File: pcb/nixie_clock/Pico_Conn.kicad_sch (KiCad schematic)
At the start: 1 part, among them U14 PicoW

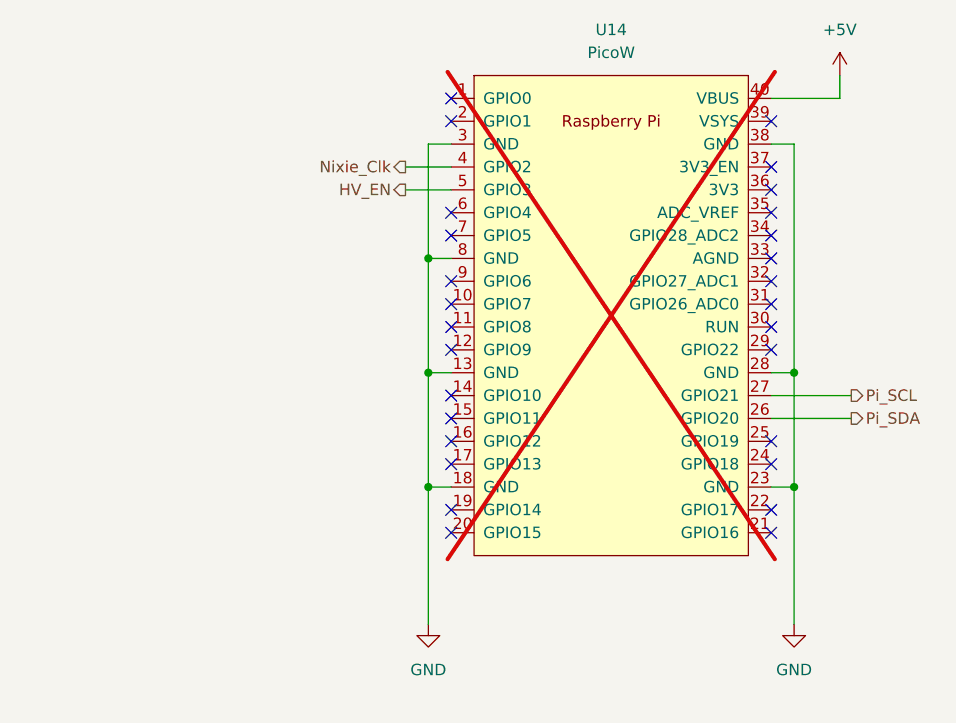
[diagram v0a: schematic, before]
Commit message: final commits before sending to jlc
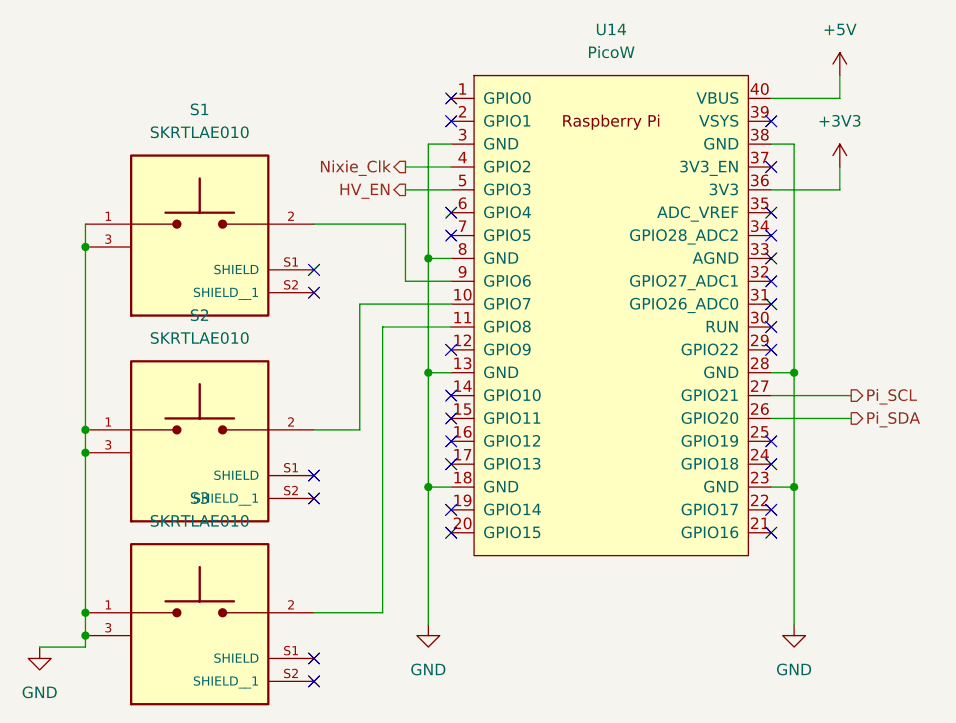
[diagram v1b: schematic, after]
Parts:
- added S1, S2, S3: SKRTLAE010, SKRTLAE010:SW_SKRTLAE010, symbol SKRTLAE010:SKRTLAE010
- U14: now fitted; now left out of the parts list
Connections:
- net GND: now also S1.1, S1.3, S2.1, S2.3, S3.1, S3.3
- net at U14.10 (GPIO7): now also S2.2
- net at U14.11 (GPIO8): now also S3.2
- net +3V3: now reaches U14.36 (3V3)
- net at U14.9 (GPIO6): now also S1.2
- no-connect marks 28 -> 30
